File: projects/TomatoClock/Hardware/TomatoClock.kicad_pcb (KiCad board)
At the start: 2 copper layers, 52.3 x 30.5 mm, 17 parts, among them J1 Boot, J2 UART, J3 USB_B_Micro, U1 STM32F103C8T6, U2 WS4518E, U3 AP1117-33, Y1 8MHz, Y2 32.768kHz

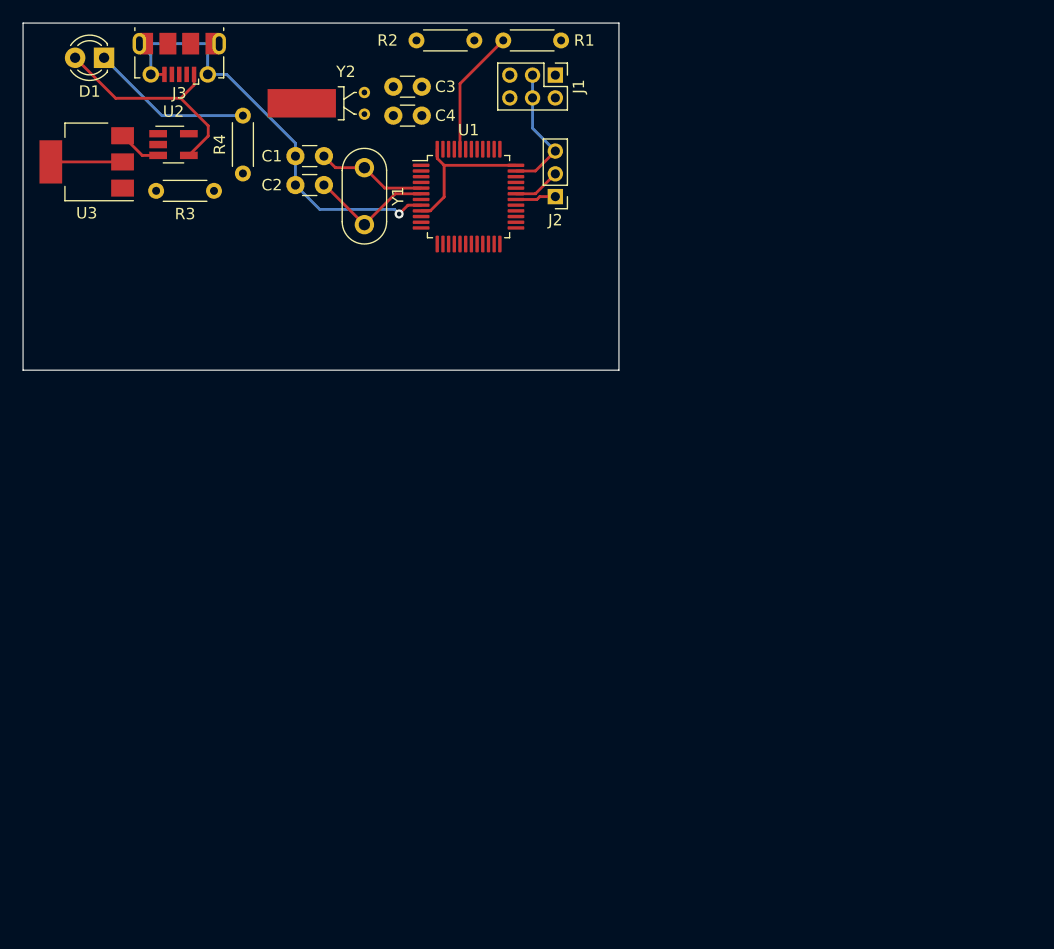
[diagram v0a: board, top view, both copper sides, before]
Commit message: TomatoClock: Update PCB and Gerber files
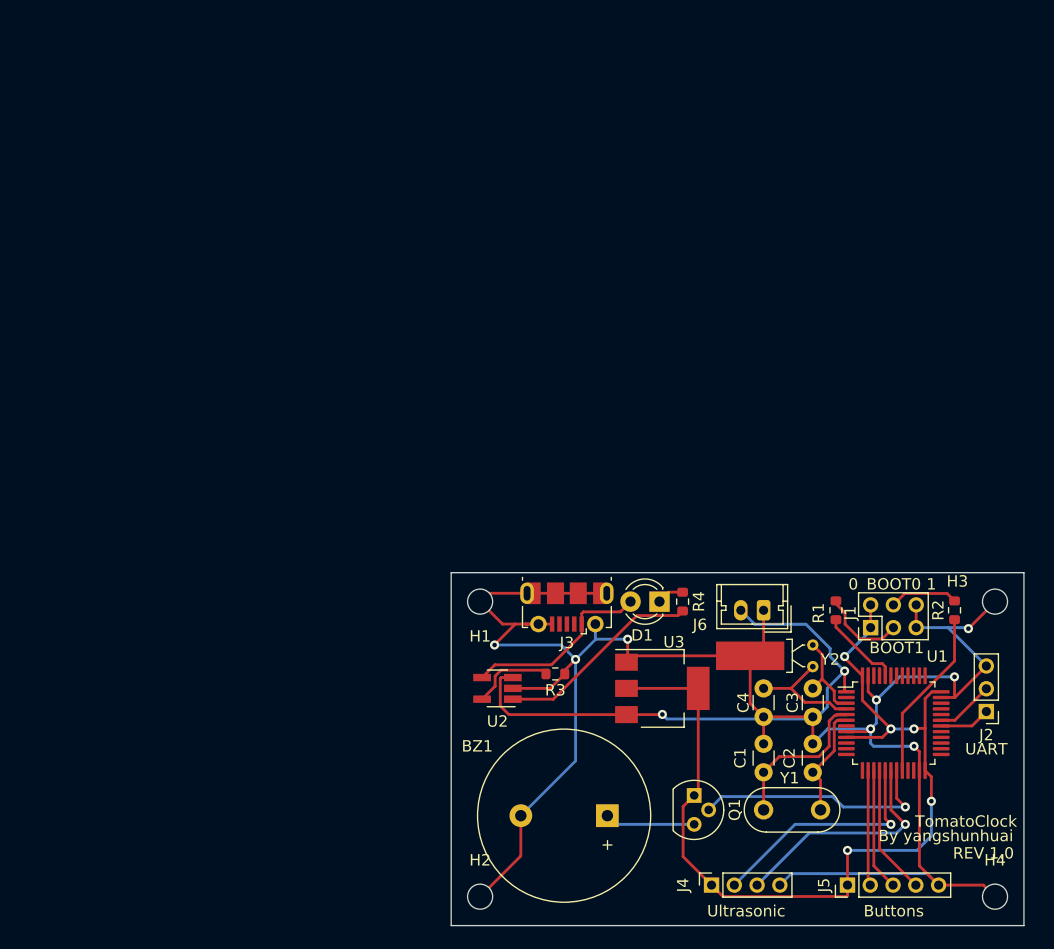
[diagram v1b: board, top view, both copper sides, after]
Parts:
- added BZ1: Buzzer, Buzzer_Beeper:Buzzer_15x7.5RM7.6, F.Cu at (84.8, 100.1)
- added H1: hole, MountingHole:MountingHole_2.2mm_M2, F.Cu at (73.7, 81.3)
- added H2: hole, MountingHole:MountingHole_2.2mm_M2, F.Cu at (73.7, 107.2)
- added H3: hole, MountingHole:MountingHole_2.2mm_M2, F.Cu at (118.9, 81.3)
- added H4: hole, MountingHole:MountingHole_2.2mm_M2, F.Cu at (118.9, 107.2)
- added J4: Ultrasonic, Connector_PinSocket_2.00mm:PinSocket_1x04_P2.00mm_Vertical, F.Cu at (94.0, 106.2)
- added J5: Buttons, Connector_PinHeader_2.00mm:PinHeader_1x05_P2.00mm_Vertical, F.Cu at (105.9, 106.2)
- added J6: Battery, Connector_Molex:Molex_Micro-Latch_53253-0270_1x02_P2.00mm_Vertical, F.Cu at (98.6, 82.0)
- added Q1: S9014, Package_TO_SOT_THT:TO-92, F.Cu at (92.5, 98.3)
- R1, R2, R3, R4: footprint Resistor_THT:R_Axial_DIN0204_L3.6mm_D1.6mm_P5.08mm_Horizontal -> Resistor_SMD:R_0603_1608Metric
- moved R2 68.8 mm to (115.3, 82.0), turned to 90 degrees
- moved U3 68.5 mm to (89.7, 88.9), turned to 0 degrees
- moved D1 68.3 mm to (89.4, 81.3)
- moved C2 67.1 mm to (102.9, 96.3), turned to 90 degrees
- moved C1 66.5 mm to (98.6, 96.3), turned to 90 degrees
- moved Y1 66.4 mm to (98.6, 99.6), turned to 0 degrees
- moved C3 64.4 mm to (102.9, 88.9), turned to 270 degrees
- moved Y2 62.5 mm to (102.9, 85.1)
- moved C4 59.9 mm to (98.6, 88.9), turned to 270 degrees
- moved U1 59.4 mm to (110.0, 91.9)
- moved J3 59.1 mm to (81.3, 81.8)
- moved J2 59.0 mm to (118.1, 90.9)
- moved R4 57.5 mm to (91.4, 81.3)
- moved J1 55.9 mm to (108.0, 83.6), turned to 90 degrees
- moved U2 55.6 mm to (75.2, 88.9), turned to 180 degrees
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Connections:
- J1 pad 2: Net-(J1-Pad2) -> +3V3
- J1 pad 3: GND -> Net-(J1-Pad3)
- J1 pad 4: GND -> Net-(J1-Pad4)
- J1 pad 5: Net-(J1-Pad5) -> GND
- J1 pad 6: +3V3 -> GND
- R1 pad 1: Net-(J1-Pad2) -> Net-(J1-Pad3)
- R2 pad 2: Net-(J1-Pad5) -> Net-(J1-Pad4)
- U1 pad 14: (no net) -> LEFT
- U1 pad 15: (no net) -> MIDDLE
- U1 pad 16: (no net) -> RIGHT
- U1 pad 17: (no net) -> US_TRIG
- U1 pad 18: (no net) -> US_ECHO
- U1 pad 19: (no net) -> BUZZER
- Y2 pad 3: (no net) -> GND
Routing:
- net GND: track 52.5 -> 179.5 mm, vias 1 -> 8
- net +3V3: track 19.6 -> 84.1 mm, vias 0 -> 5
- net +BATT: track 3.83 -> 50.6 mm, vias 0 -> 2
- net BUZZER: track 0.00 -> 21.7 mm, vias 0 -> 1
- net US_TRIG: track 0.00 -> 20.9 mm, vias 0 -> 1
- net US_ECHO: track 0.00 -> 20.5 mm, vias 0 -> 1
- net Net-(R4-Pad2): track 0.00 -> 18.1 mm
- net BOOT1: track 0.00 -> 15.1 mm
- net Net-(D1-Pad1): track 14.3 -> 2.37 mm
- net RIGHT: track 0.00 -> 11.4 mm
- net MIDDLE: track 0.00 -> 10.8 mm
- net Net-(C4-Pad1): track 0.00 -> 10.7 mm
- net LEFT: track 0.00 -> 10.1 mm
- net Net-(C3-Pad1): track 0.00 -> 7.97 mm
- net Net-(BZ1-Pad1): track 0.00 -> 7.94 mm
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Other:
- board size 52.3 x 30.5 mm -> 50.3 x 31 mm
- board text added: "0"
- board text added: "1"
- board text added: "BOOT0"
- board text added: "BOOT1"
- board text added: "Buttons"
- board text added: "By yangshunhuai"
- board text added: "REV 1.0"
- board text added: "TomatoClock"
- board text added: "UART"
- board text added: "Ultrasonic"
